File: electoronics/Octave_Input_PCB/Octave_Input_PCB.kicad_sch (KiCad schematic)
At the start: 28 parts, among them SW1 SW_Hot_Swap_Socket, SW10 SW_Hot_Swap_Socket, SW11 SW_Hot_Swap_Socket, SW12 SW_Hot_Swap_Socket, SW13 SW_Hot_Swap_Socket, SW14 SW_Hot_Swap_Socket, SW2 SW_Hot_Swap_Socket, SW3 SW_Hot_Swap_Socket, SW4 SW_Hot_Swap_Socket, SW5 SW_Hot_Swap_Socket, SW6 SW_Hot_Swap_Socket, SW7 SW_Hot_Swap_Socket, SW8 SW_Hot_Swap_Socket, SW9 SW_Hot_Swap_Socket

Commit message: Update schematic and PCB
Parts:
- D1, D10, D11, D12, D13, D14, D2, D3, D4, D5, D6, D7, D8, D9: footprint Diode_SMD:D_SOD-323 -> Octave_Library:D_SOD-323
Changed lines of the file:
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@@
       (effects (font (size 1.27 1.27)) (justify right))
     )
-    (property "Footprint" "Diode_SMD:D_SOD-323" (id 2) (at 120.015 78.74 0)
+    (property "Footprint" "Octave_Library:D_SOD-323" (id 2) (at 120.015 78.74 0)
       (effects (font (size 1.27 1.27)) hide)
     )
@@
       (effects (font (size 1.27 1.27)) (justify right))
     )
-    (property "Footprint" "Diode_SMD:D_SOD-323" (id 2) (at 104.775 78.74 0)
+    (property "Footprint" "Octave_Library:D_SOD-323" (id 2) (at 104.775 78.74 0)
       (effects (font (size 1.27 1.27)) hide)
     )
@@
       (effects (font (size 1.27 1.27)) (justify right))
     )
-    (property "Footprint" "Diode_SMD:D_SOD-323" (id 2) (at 120.015 114.3 0)
+    (property "Footprint" "Octave_Library:D_SOD-323" (id 2) (at 120.015 114.3 0)
       (effects (font (size 1.27 1.27)) hide)
     )
@@
       (effects (font (size 1.27 1.27)) (justify right))
     )
-    (property "Footprint" "Diode_SMD:D_SOD-323" (id 2) (at 104.775 60.96 0)
+    (property "Footprint" "Octave_Library:D_SOD-323" (id 2) (at 104.775 60.96 0)
       (effects (font (size 1.27 1.27)) hide)
     )
@@
       (effects (font (size 1.27 1.27)) (justify right))
     )
-    (property "Footprint" "Diode_SMD:D_SOD-323" (id 2) (at 89.535 78.74 0)
+    (property "Footprint" "Octave_Library:D_SOD-323" (id 2) (at 89.535 78.74 0)
       (effects (font (size 1.27 1.27)) hide)
     )
@@
       (effects (font (size 1.27 1.27)) (justify right))
     )
-    (property "Footprint" "Diode_SMD:D_SOD-323" (id 2) (at 89.535 60.96 0)
+    (property "Footprint" "Octave_Library:D_SOD-323" (id 2) (at 89.535 60.96 0)
       (effects (font (size 1.27 1.27)) hide)
     )
@@
       (effects (font (size 1.27 1.27)) (justify right))
     )
-    (property "Footprint" "Diode_SMD:D_SOD-323" (id 2) (at 74.295 78.74 0)
+    (property "Footprint" "Octave_Library:D_SOD-323" (id 2) (at 74.295 78.74 0)
       (effects (font (size 1.27 1.27)) hide)
     )
@@
       (effects (font (size 1.27 1.27)) (justify right))
     )
-    (property "Footprint" "Diode_SMD:D_SOD-323" (id 2) (at 89.535 96.52 0)
+    (property "Footprint" "Octave_Library:D_SOD-323" (id 2) (at 89.535 96.52 0)
       (effects (font (size 1.27 1.27)) hide)
     )
@@
       (effects (font (size 1.27 1.27)) (justify right))
     )
-    (property "Footprint" "Diode_SMD:D_SOD-323" (id 2) (at 74.295 60.96 0)
+    (property "Footprint" "Octave_Library:D_SOD-323" (id 2) (at 74.295 60.96 0)
       (effects (font (size 1.27 1.27)) hide)
     )
@@
       (effects (font (size 1.27 1.27)) (justify right))
     )
-    (property "Footprint" "Diode_SMD:D_SOD-323" (id 2) (at 74.295 96.52 0)
+    (property "Footprint" "Octave_Library:D_SOD-323" (id 2) (at 74.295 96.52 0)
       (effects (font (size 1.27 1.27)) hide)
     )
@@
       (effects (font (size 1.27 1.27)) (justify right))
     )
-    (property "Footprint" "Diode_SMD:D_SOD-323" (id 2) (at 120.015 96.52 0)
+    (property "Footprint" "Octave_Library:D_SOD-323" (id 2) (at 120.015 96.52 0)
       (effects (font (size 1.27 1.27)) hide)
     )
@@
       (effects (font (size 1.27 1.27)) (justify right))
     )
-    (property "Footprint" "Diode_SMD:D_SOD-323" (id 2) (at 104.775 96.52 0)
+    (property "Footprint" "Octave_Library:D_SOD-323" (id 2) (at 104.775 96.52 0)
       (effects (font (size 1.27 1.27)) hide)
     )
@@
       (effects (font (size 1.27 1.27)) (justify right))
     )
-    (property "Footprint" "Diode_SMD:D_SOD-323" (id 2) (at 74.295 114.3 0)
+    (property "Footprint" "Octave_Library:D_SOD-323" (id 2) (at 74.295 114.3 0)
       (effects (font (size 1.27 1.27)) hide)
     )
@@
       (effects (font (size 1.27 1.27)) (justify right))
     )
-    (property "Footprint" "Diode_SMD:D_SOD-323" (id 2) (at 120.015 60.96 0)
+    (property "Footprint" "Octave_Library:D_SOD-323" (id 2) (at 120.015 60.96 0)
       (effects (font (size 1.27 1.27)) hide)
     )
@@
   (symbol_instances
     (path "/709f02fa-f113-4f34-aada-ad74ed9e0d25"
-      (reference "D1") (unit 1) (value "1N4148WS") (footprint "Diode_SMD:D_SOD-323")
+      (reference "D1") (unit 1) (value "1N4148WS") (footprint "Octave_Library:D_SOD-323")
     )
     (path "/3c5d03ad-ef2a-44d3-bc52-83fc5cd731c2"
-      (reference "D2") (unit 1) (value "1N4148WS") (footprint "Diode_SMD:D_SOD-323")
+      (reference "D2") (unit 1) (value "1N4148WS") (footprint "Octave_Library:D_SOD-323")
     )
     (path "/1a8ff821-98c8-41ef-919b-9109469cd4f0"
-      (reference "D3") (unit 1) (value "1N4148WS") (footprint "Diode_SMD:D_SOD-323")
+      (reference "D3") (unit 1) (value "1N4148WS") (footprint "Octave_Library:D_SOD-323")
     )
     (path "/fbe8ce2d-ce37-4567-b78b-14cbdd8d5fa9"
-      (reference "D4") (unit 1) (value "1N4148WS") (footprint "Diode_SMD:D_SOD-323")
+      (reference "D4") (unit 1) (value "1N4148WS") (footprint "Octave_Library:D_SOD-323")
     )
     (path "/4180a1a8-8e9e-403c-882e-e605ec012797"
-      (reference "D5") (unit 1) (value "1N4148WS") (footprint "Diode_SMD:D_SOD-323")
+      (reference "D5") (unit 1) (value "1N4148WS") (footprint "Octave_Library:D_SOD-323")
     )
     (path "/289a3e37-e58b-4925-9d57-18405effc2cb"
-      (reference "D6") (unit 1) (value "1N4148WS") (footprint "Diode_SMD:D_SOD-323")
+      (reference "D6") (unit 1) (value "1N4148WS") (footprint "Octave_Library:D_SOD-323")
     )
     (path "/0e2cc3b9-7e96-4254-8233-44f8db422f6e"
-      (reference "D7") (unit 1) (value "1N4148WS") (footprint "Diode_SMD:D_SOD-323")
+      (reference "D7") (unit 1) (value "1N4148WS") (footprint "Octave_Library:D_SOD-323")
     )
     (path "/053dae26-0d29-4615-8f3a-499ae7356113"
-      (reference "D8") (unit 1) (value "1N4148WS") (footprint "Diode_SMD:D_SOD-323")
+      (reference "D8") (unit 1) (value "1N4148WS") (footprint "Octave_Library:D_SOD-323")
     )
     (path "/764ac2d4-e593-4865-97ff-ed8b82b2353d"
-      (reference "D9") (unit 1) (value "1N4148WS") (footprint "Diode_SMD:D_SOD-323")
+      (reference "D9") (unit 1) (value "1N4148WS") (footprint "Octave_Library:D_SOD-323")
     )
     (path "/58bc63e9-f591-47dd-8596-d72edc57116c"
-      (reference "D10") (unit 1) (value "1N4148WS") (footprint "Diode_SMD:D_SOD-323")
+      (reference "D10") (unit 1) (value "1N4148WS") (footprint "Octave_Library:D_SOD-323")
     )
     (path "/9caea4a2-5bc1-44cc-8293-300131386895"
-      (reference "D11") (unit 1) (value "1N4148WS") (footprint "Diode_SMD:D_SOD-323")
+      (reference "D11") (unit 1) (value "1N4148WS") (footprint "Octave_Library:D_SOD-323")
     )
     (path "/870e1d5b-9785-4c66-8095-64350a305b0a"
-      (reference "D12") (unit 1) (value "1N4148WS") (footprint "Diode_SMD:D_SOD-323")
+      (reference "D12") (unit 1) (value "1N4148WS") (footprint "Octave_Library:D_SOD-323")
     )
     (path "/fbc0e23d-9856-4676-a4d7-95fcc2785fe2"
-      (reference "D13") (unit 1) (value "1N4148WS") (footprint "Diode_SMD:D_SOD-323")
+      (reference "D13") (unit 1) (value "1N4148WS") (footprint "Octave_Library:D_SOD-323")
     )
     (path "/15dd2ce1-5057-4d96-93de-f9436edad95a"
-      (reference "D14") (unit 1) (value "1N4148WS") (footprint "Diode_SMD:D_SOD-323")
+      (reference "D14") (unit 1) (value "1N4148WS") (footprint "Octave_Library:D_SOD-323")
     )
     (path "/ec285e65-9c46-4fa7-bf57-be16d5aaed04"

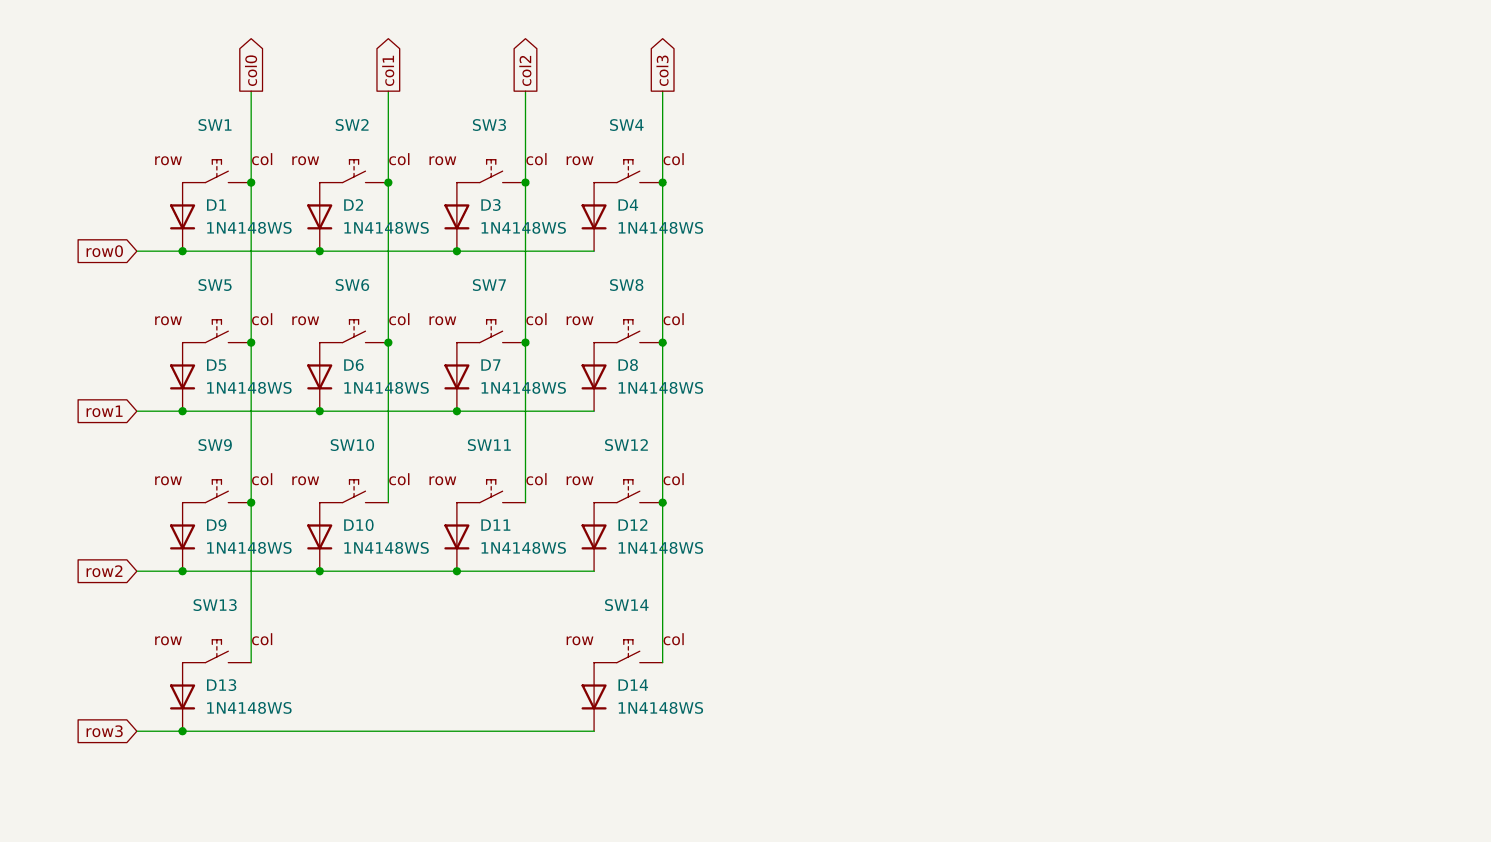
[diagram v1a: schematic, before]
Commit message: Update schematic
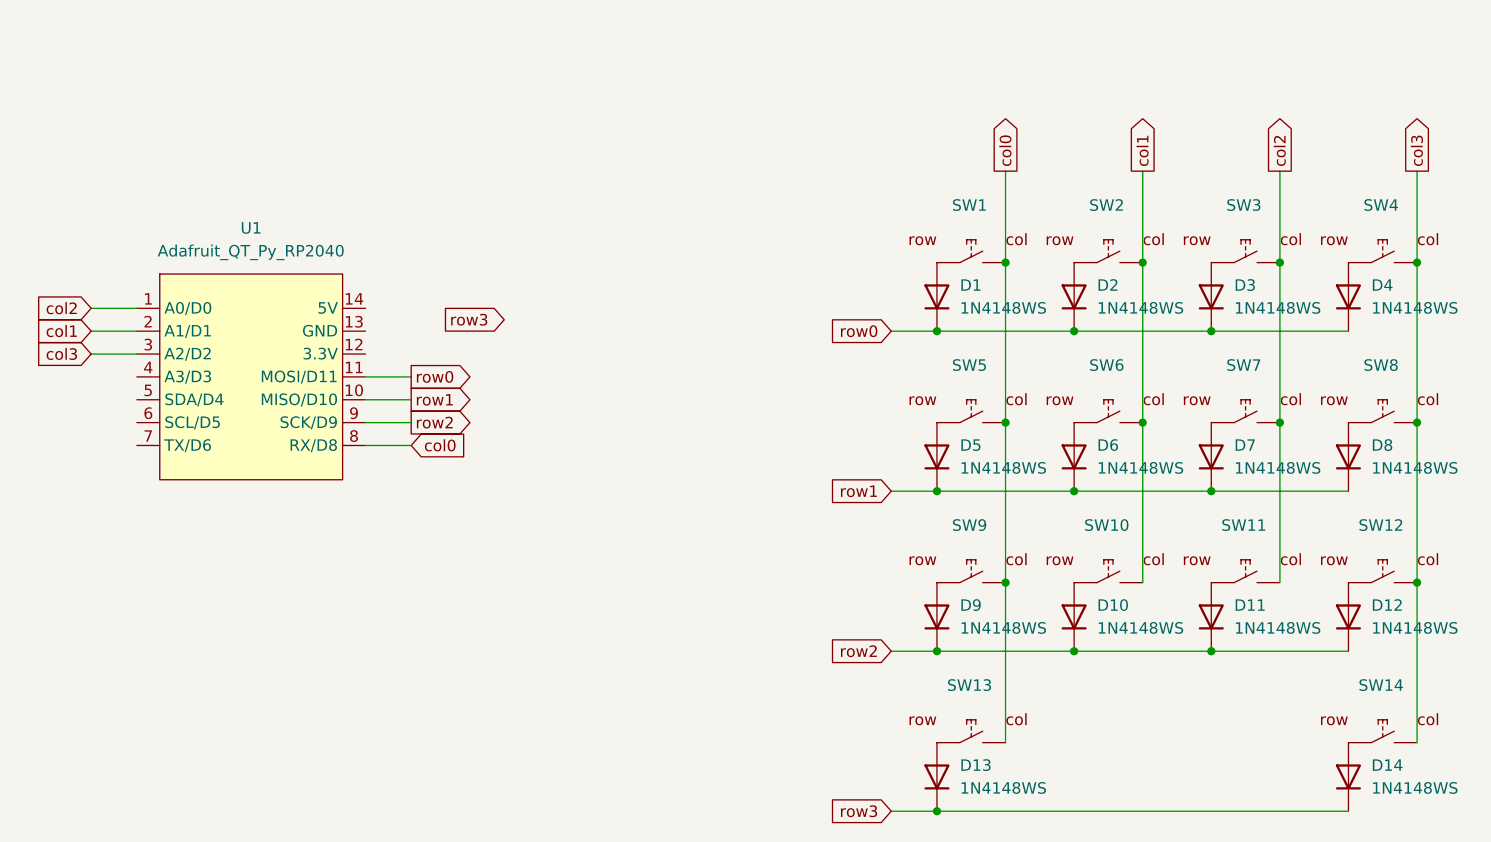
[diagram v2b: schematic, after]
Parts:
- added U1: Adafruit_QT_Py_RP2040, Octave_Library:Adafruit_QT_Py_RP2040, symbol Octave_Library:Adafruit_QT_Py_RP2040
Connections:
- net col0: now also U1.8 (RX/D8)
- net col1: now also U1.2 (A1/D1)
- net col2: now also U1.1 (A0/D0)
- net col3: now also U1.3 (A2/D2)
- net row0: now also U1.11 (MOSI/D11)
- net row1: now also U1.10 (MISO/D10)
- net row2: now also U1.9 (SCK/D9)
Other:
- moved on the sheet: D1, D10, D11, D12, D13, D14, D2, D3, D4, D5, D6, D7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
